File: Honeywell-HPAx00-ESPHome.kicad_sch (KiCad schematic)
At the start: 25 parts, among them J1 Conn_01x06, J2 Conn_01x01, J3 Conn_01x01, J4 Conn_01x01, J5 Conn_01x01, J6 Conn_01x01, J7 Conn_01x01, U1 mini_esp32

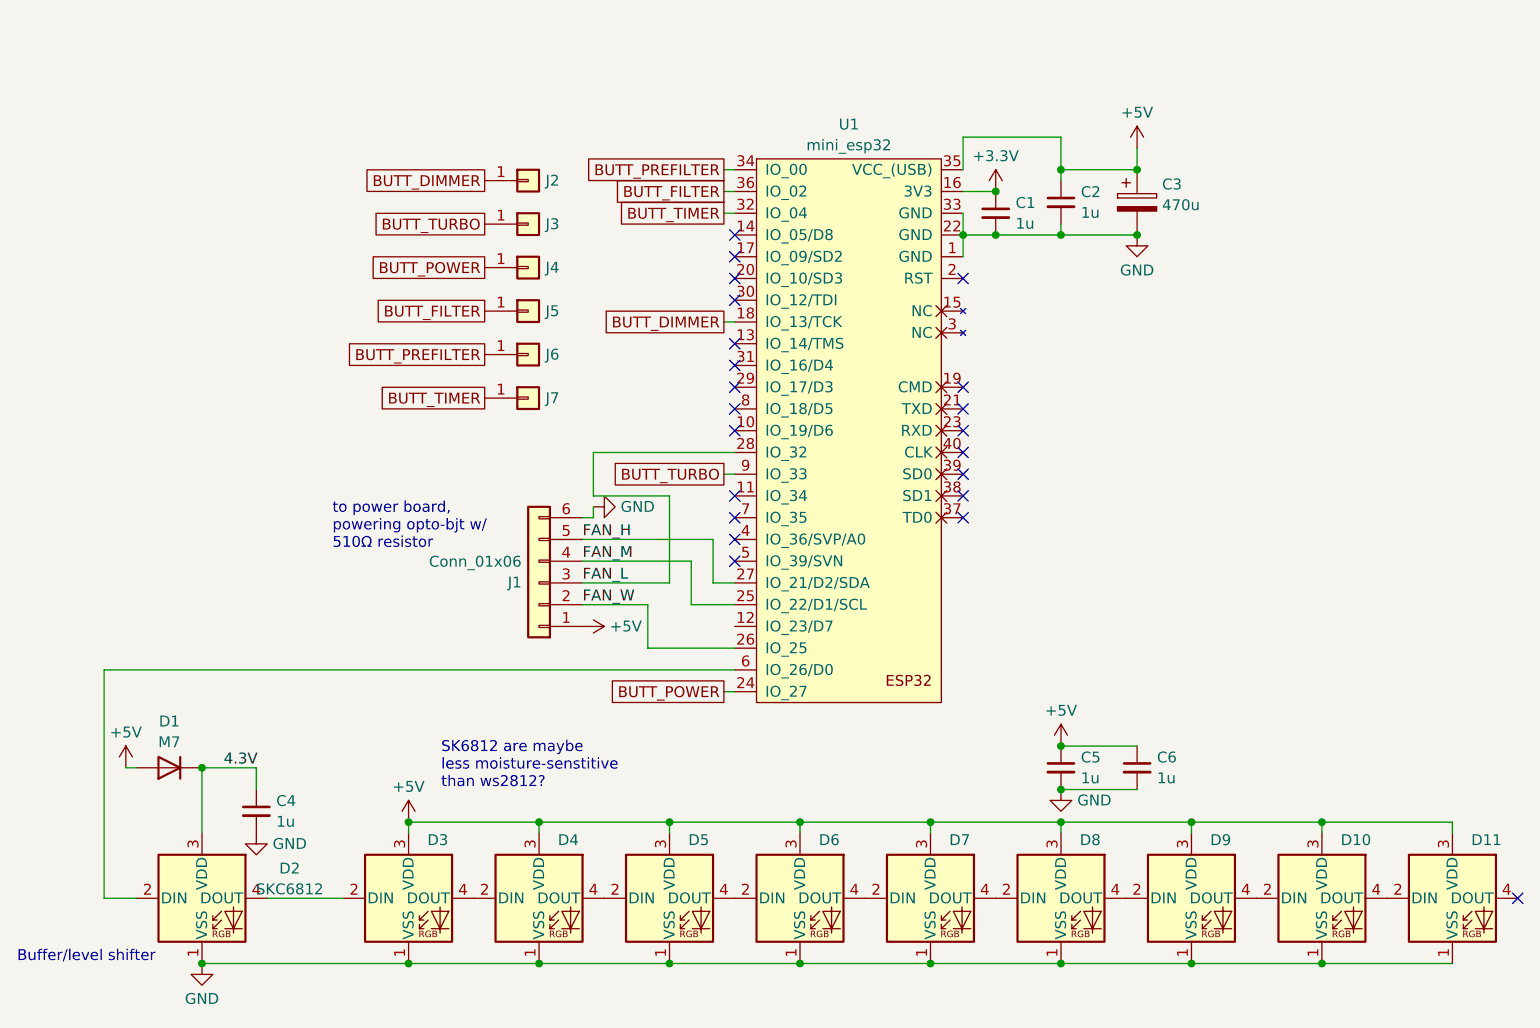
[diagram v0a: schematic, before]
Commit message: Update design
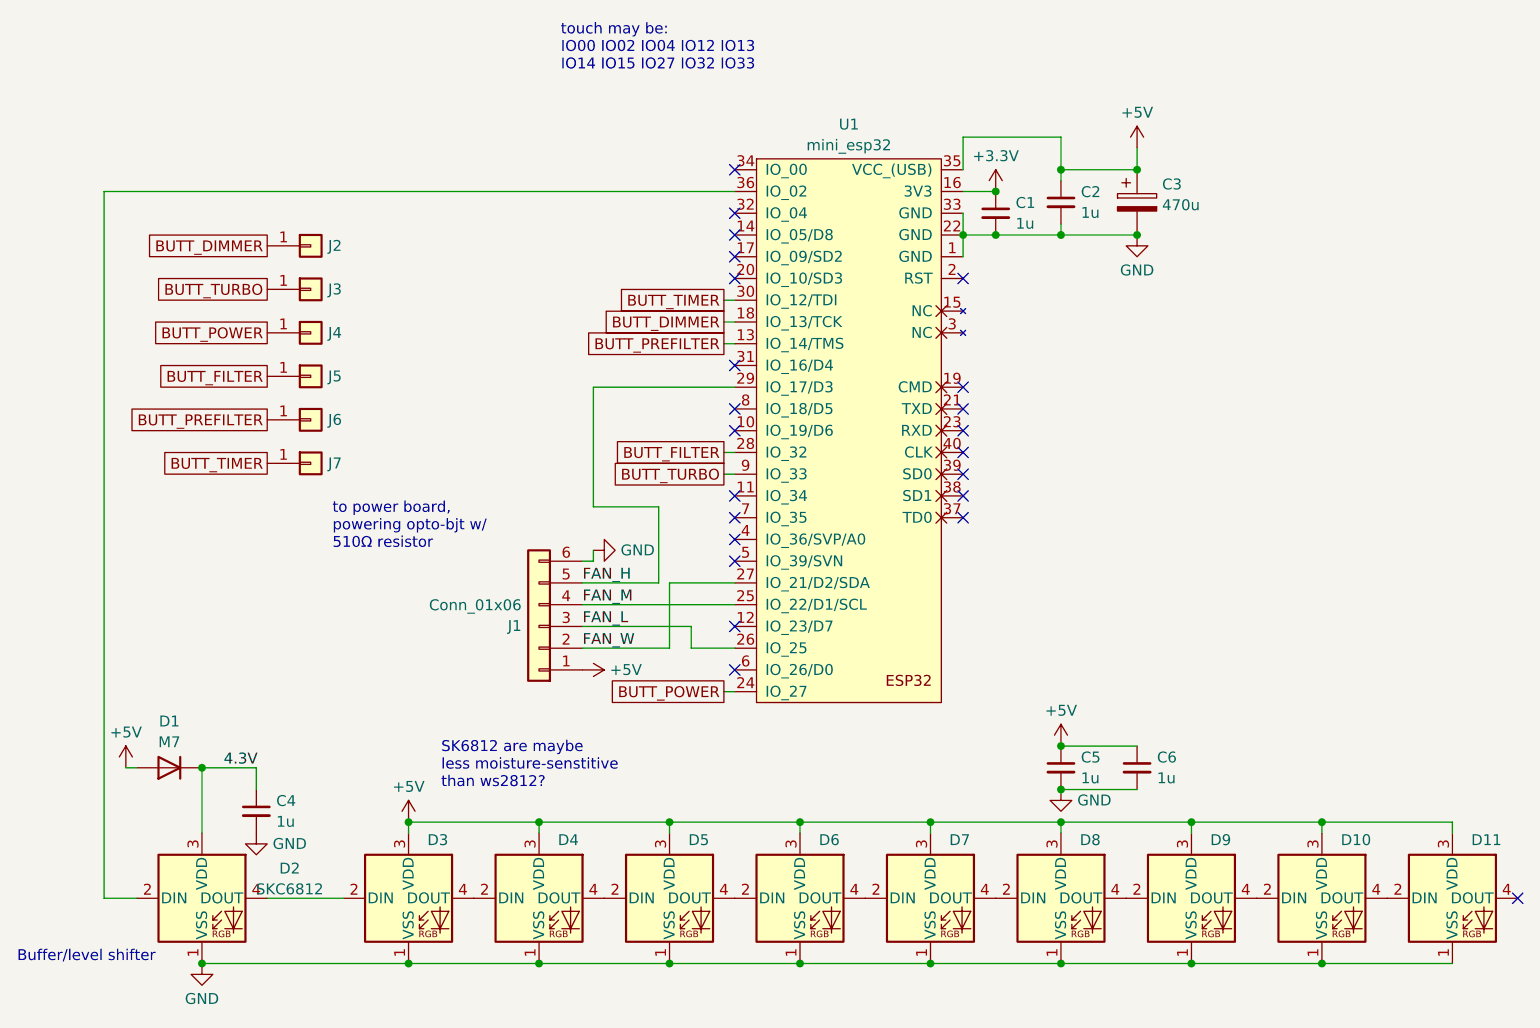
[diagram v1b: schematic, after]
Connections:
- net BUTT_FILTER: now also U1.28 (IO_32); no longer U1.36 (IO_02)
- net BUTT_PREFILTER: now also U1.13 (IO_14/TMS); no longer U1.34 (IO_00)
- net BUTT_TIMER: now also U1.30 (IO_12/TDI); no longer U1.32 (IO_04)
- net FAN_H: now also U1.29 (IO_17/D3); no longer U1.27 (IO_21/D2/SDA)
- net FAN_L: now also U1.26 (IO_25); no longer U1.28 (IO_32)
- net FAN_W: now also U1.27 (IO_21/D2/SDA); no longer U1.26 (IO_25)
- net at D2.2 (DIN): now also U1.36 (IO_02); no longer U1.6 (IO_26/D0)
- no-connect marks 22 -> 23
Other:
- note added: "touch may be: IO00 IO02 IO04 IO12 IO13 IO14 IO15 IO27 IO32 IO33"
- moved on the sheet: J1, J2, J3, J4, J5, J6, J7

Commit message: final tweaks
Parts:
- J2, J3, J4, J5, J6, J7: footprint TestPoint:TestPoint_THTPad_D1.5mm_Drill0.7mm -> TestPoint:TestPoint_THTPad_D2.0mm_Drill1.0mm
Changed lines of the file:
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@@
       (effects (font (size 1.27 1.27)) (justify left) hide)
     )
-    (property "Footprint" "TestPoint:TestPoint_THTPad_D1.5mm_Drill0.7mm" (at 96.52 82.55 0)
+    (property "Footprint" "TestPoint:TestPoint_THTPad_D2.0mm_Drill1.0mm" (at 96.52 82.55 0)
       (effects (font (size 1.27 1.27)) hide)
     )
@@
       (effects (font (size 1.27 1.27)) (justify left) hide)
     )
-    (property "Footprint" "TestPoint:TestPoint_THTPad_D1.5mm_Drill0.7mm" (at 96.52 87.63 0)
+    (property "Footprint" "TestPoint:TestPoint_THTPad_D2.0mm_Drill1.0mm" (at 96.52 87.63 0)
       (effects (font (size 1.27 1.27)) hide)
     )
@@
       (effects (font (size 1.27 1.27)) (justify left) hide)
     )
-    (property "Footprint" "TestPoint:TestPoint_THTPad_D1.5mm_Drill0.7mm" (at 96.52 62.23 0)
+    (property "Footprint" "TestPoint:TestPoint_THTPad_D2.0mm_Drill1.0mm" (at 96.52 62.23 0)
       (effects (font (size 1.27 1.27)) hide)
     )
@@
       (effects (font (size 1.27 1.27)) (justify left) hide)
     )
-    (property "Footprint" "TestPoint:TestPoint_THTPad_D1.5mm_Drill0.7mm" (at 96.52 77.47 0)
+    (property "Footprint" "TestPoint:TestPoint_THTPad_D2.0mm_Drill1.0mm" (at 96.52 77.47 0)
       (effects (font (size 1.27 1.27)) hide)
     )
@@
       (effects (font (size 1.27 1.27)) (justify left) hide)
     )
-    (property "Footprint" "TestPoint:TestPoint_THTPad_D1.5mm_Drill0.7mm" (at 96.52 72.39 0)
+    (property "Footprint" "TestPoint:TestPoint_THTPad_D2.0mm_Drill1.0mm" (at 96.52 72.39 0)
       (effects (font (size 1.27 1.27)) hide)
     )
@@
       (effects (font (size 1.27 1.27)) (justify left) hide)
     )
-    (property "Footprint" "TestPoint:TestPoint_THTPad_D1.5mm_Drill0.7mm" (at 96.52 67.31 0)
-      (effects (font (size 1.27 1.27)) hide)
-    )
+    (property "Footprint" "TestPoint:TestPoint_THTPad_D2.0mm_Drill1.0mm" (at 96.52 67.31 0)
+      (effects (font (size 1.27 1.27)) hide)
+    )
